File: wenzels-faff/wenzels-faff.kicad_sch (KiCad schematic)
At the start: 139 parts, among them J1 9V-18V, J2 In, J3 Out, Q1 NPN, Q2 NPN, Q3 NPN, Q4 NPN, Q5 J113, Q6 J113, U1 TL084, U2 TL072

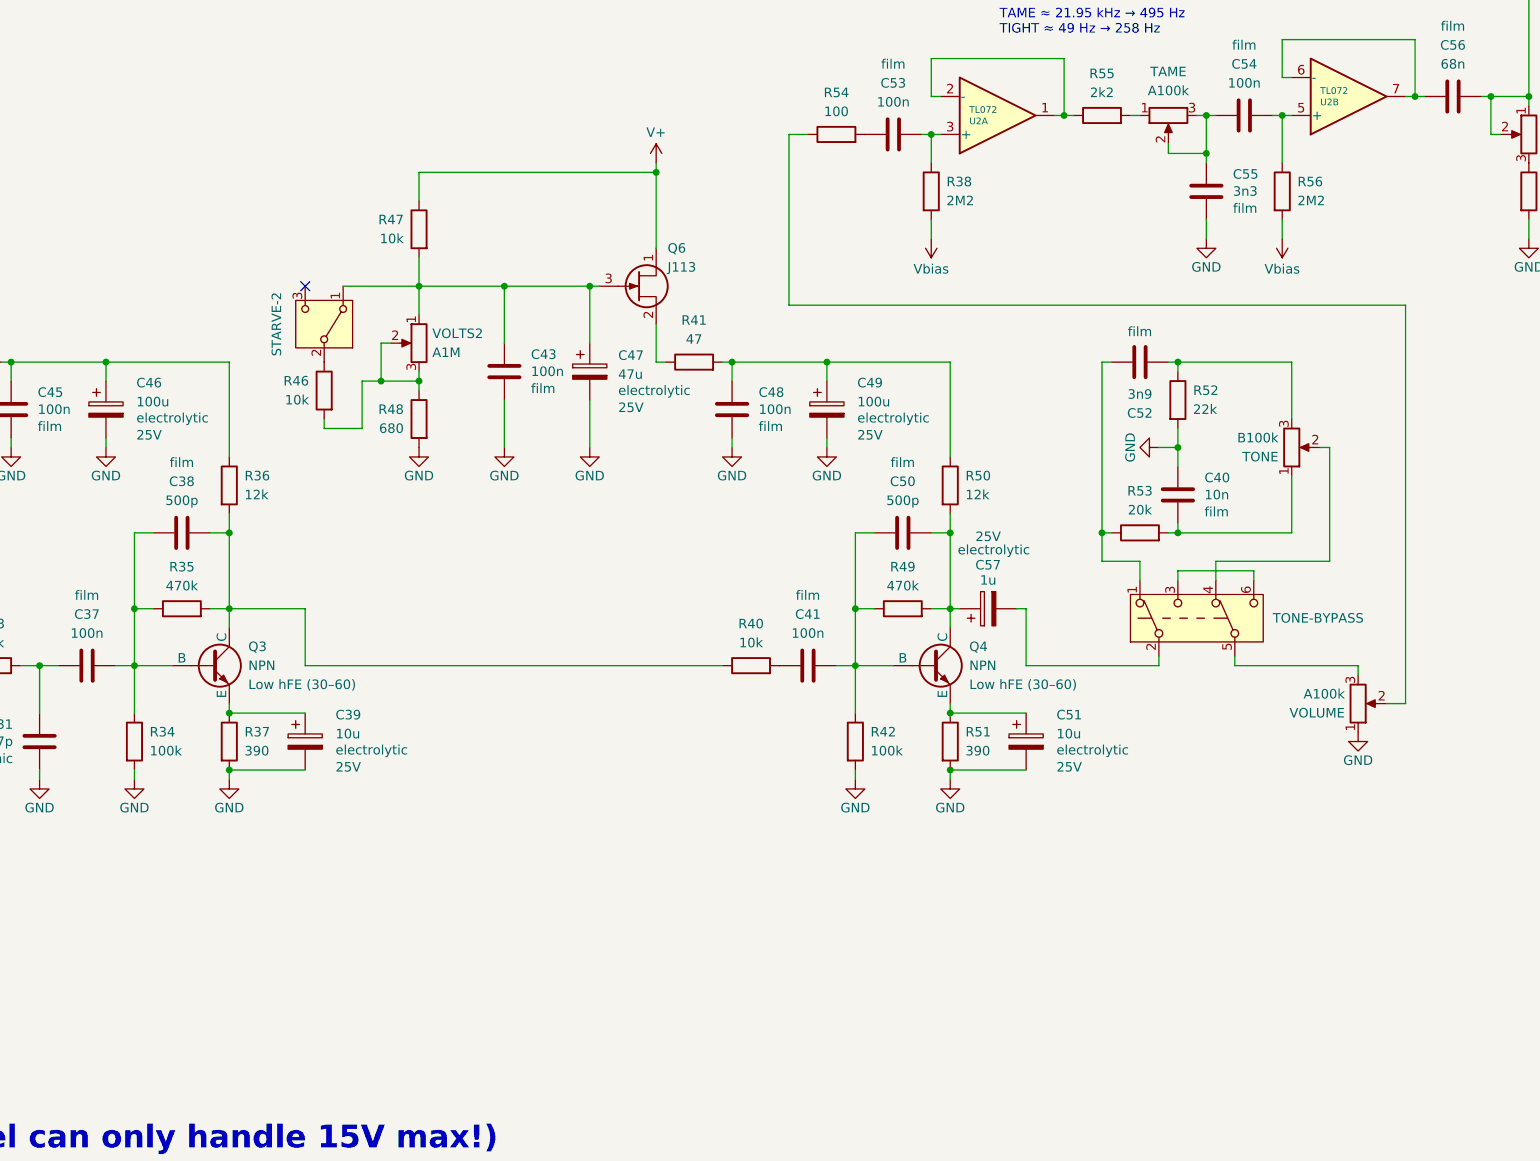
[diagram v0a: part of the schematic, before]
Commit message: wenzels-faff release-2026-09-r2
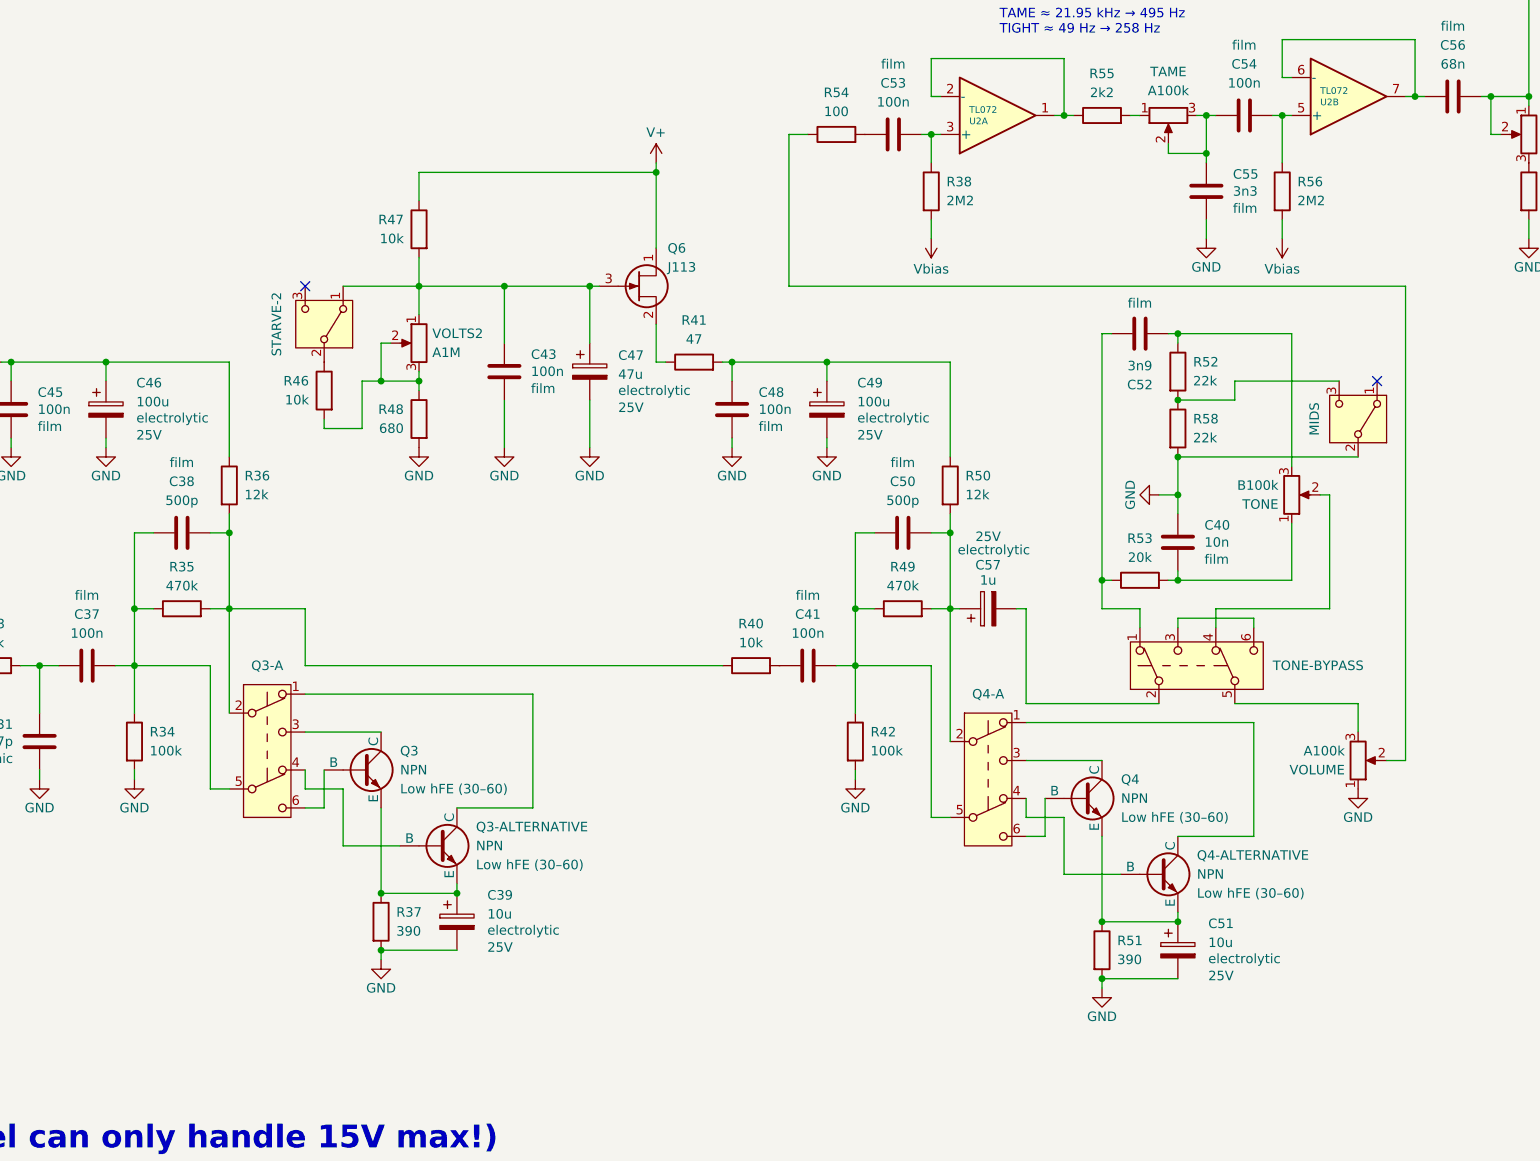
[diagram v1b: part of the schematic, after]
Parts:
- added MIDS: SW_SPDT, symbol Switch:SW_SPDT
- added Q3-A, Q4-A: SW_Push_DPDT, symbol Switch:SW_Push_DPDT
- added Q3-ALTERNATIVE, Q4-ALTERNATIVE: NPN, symbol Simulation_SPICE:NPN
- added R58: 22k, symbol Device:R
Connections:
- net GND: now also MIDS.2 (B), R58.2; no longer R52.2
- net at C41.2, C50.1, R42.1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: now also Q4-A.5 (B); no longer Q4.2 (B)
- net at C50.2, C57.1, R49.2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: now also Q4-A.2 (B); no longer Q4.1 (C)
- net at C37.2, C38.1, R34.1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: now also Q3-A.5 (B); no longer Q3.2 (B)
- net at C38.2, R35.2, R36.2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: now also Q3-A.2 (B); no longer Q3.1 (C)
- net at C39.1, Q3.3 (E), R37.1: now also Q3-ALTERNATIVE.3 (E)
- net at C51.1, Q4.3 (E), R51.1: now also Q4-ALTERNATIVE.3 (E)
- new net: Q4-A.1 (A), Q4-ALTERNATIVE.1 (C)
- new net: Q4-A.4 (A), Q4-ALTERNATIVE.2 (B)
- new net: Q4-A.3 (C), Q4.1 (C)
- new net: Q4-A.6 (C), Q4.2 (B)
- new net: Q3-A.1 (A), Q3-ALTERNATIVE.1 (C)
- new net: Q3-A.4 (A), Q3-ALTERNATIVE.2 (B)
- new net: Q3-A.3 (C), Q3.1 (C)
- new net: Q3-A.6 (C), Q3.2 (B)
- new net: MIDS.3 (C), R52.2, R58.1
- no-connect marks 2 -> 3
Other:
- moved on the sheet: C39, C40, C52, Q3, R37, R52, R53, TONE, TONE-BYPASS, VOLUME
